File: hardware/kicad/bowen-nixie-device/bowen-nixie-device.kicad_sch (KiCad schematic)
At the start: 122 parts, among them J1 Conn_01x02_Pin, J2 Conn_01x02_Pin, J3 Conn_01x04_Pin, J4 Qwiic/Stemma QT, J5 Conn_01x03_Pin, Q1 MMBTA42, Q10 MMBTA42, Q11 MMBTA42, Q12 MMBTA42, Q13 MMBTA42, Q14 MMBTA42, Q15 MMBTA42, Q16 MMBTA42, Q17 MMBTA42, Q18 MMBTA42, Q19 MMBTA42, Q2 MMBTA92, Q20 MMBTA42, Q21 MMBTA42, Q22 MMBTA42, Q23 MMBTA42, Q24 MMBTA42, Q25 MMBTA42, Q26 MMBTA42, Q27 MMBTA42, Q28 MMBTA42, Q29 MMBTA42, Q3 MMBTA42, Q30 MMBTA42, Q31 MMBTA42, Q32 MMBTA42, Q33 MMBTA42, Q34 MMBTA42, Q35 MMBTA42, Q36 MMBTA42, Q37 MMBTA42, Q38 MMBTA42, Q39 MMBTA42, Q4 MMBTA92, Q40 MMBTA42, Q41 MMBTA42, Q42 MMBTA42, Q43 MMBTA42, Q44 MMBTA42, Q45 MMBTA42, Q46 MMBTA42, Q47 MMBTA42, Q48 MMBTA42, Q5 MMBTA42, Q6 MMBTA92, Q7 MMBTA42, Q8 MMBTA92, Q9 MMBTA42, U1 MOUDLE-SEEEDUINO-XIAO-ESP32C3, U11 NCH8200HV, U12 DS3231, U2 74HC595, U3 74HC595, U4 74HC595, U5 74HC595, U6 74HC595

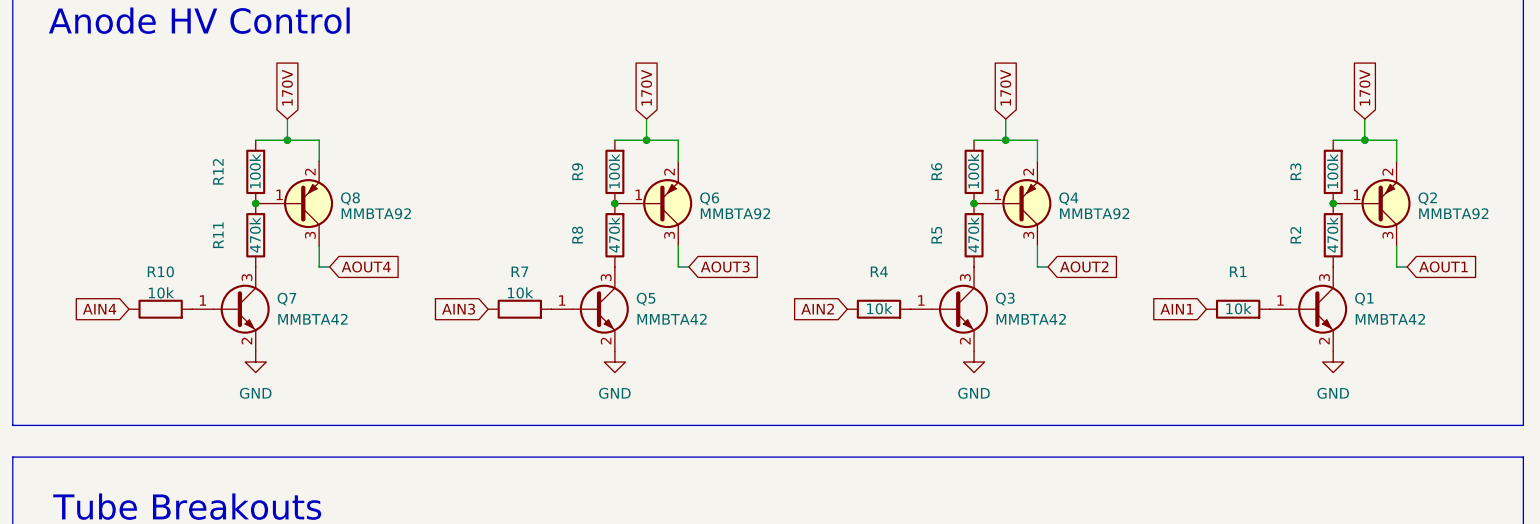
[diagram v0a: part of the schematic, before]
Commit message: bowen fixes, final v1
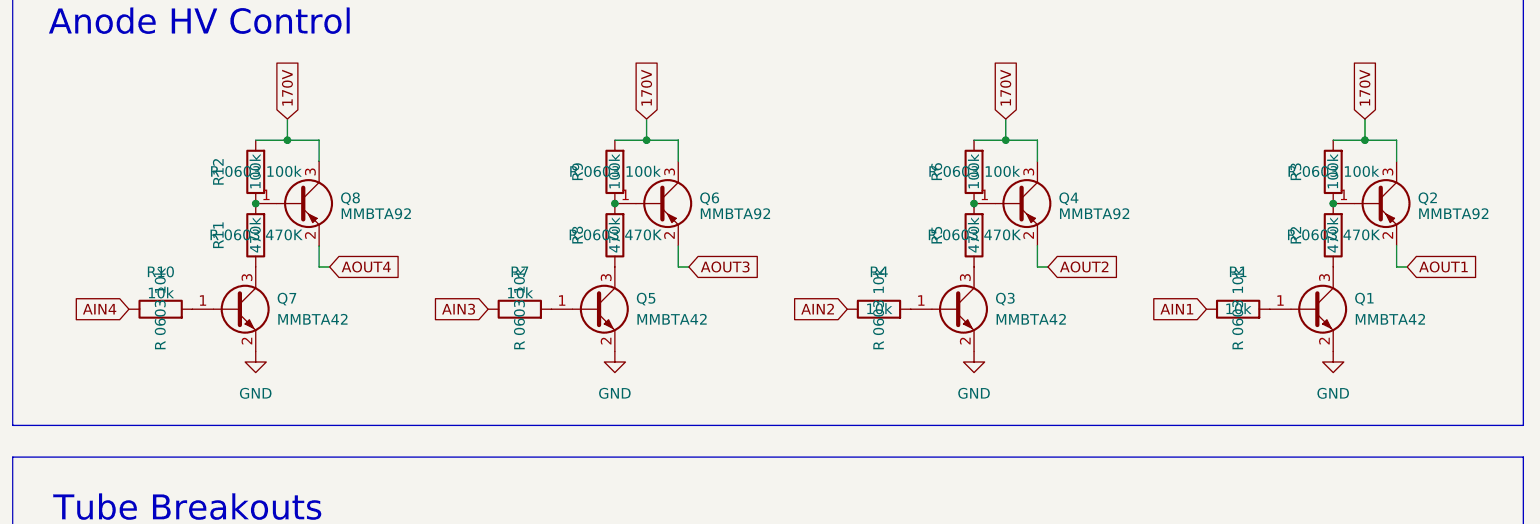
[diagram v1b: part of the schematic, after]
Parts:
- J4: MPN (none) -> BM04B-SRSS-TB
- Q1, Q10, Q11, Q12, Q13, Q14, Q15, Q16, Q17, Q18, Q19, Q20, Q21, Q22, Q23, Q24, Q25, Q26, Q27, Q28, Q29, Q3, Q30, Q31, Q32, Q33, Q34, Q35, Q36, Q37, Q38, Q39, Q40, Q41, Q42, Q43, Q44, Q45, Q46, Q47, Q48, Q5, Q7, Q9: MPN (none) -> MMBTA42LT1G; Package (none) -> SOT-23
- Q2, Q4, Q6, Q8: footprint PCM_Package_TO_SOT_SMD_AKL:SOT-23 -> Package_TO_SOT_SMD:SOT-23; symbol PCM_Transistor_BJT_AKL:MMBTA92 -> Transistor_BJT:MMBTA92; MPN (none) -> MMBTA92LT1G; Package (none) -> SOT-23
- R1, R10, R13, R14, R15, R16, R17, R18, R19, R20, R21, R22, R23, R24, R25, R26, R27, R28, R29, R30, R31, R32, R33, R34, R35, R36, R37, R38, R39, R4, R40, R41, R42, R43, R44, R45, R46, R47, R48, R49, R50, R51, R52, R7: MPN (none) -> RC0603JR-0710KL; Package (none) -> 0603
- R11, R2, R5, R8: MPN (none) -> RC1206FR-07470KL; Package (none) -> 1206
- R12, R3, R6, R9: MPN (none) -> RC0402FR-07100KL; Package (none) -> 0603
- U11: now in the parts list
- U2, U3, U4, U5, U6: MPN (none) -> 74HC595D; Package (none) -> SOIC-16
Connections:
- net 170V: now also Q2.3 (C), Q4.3 (C), Q6.3 (C), Q8.3 (C); no longer Q2.2 (E), Q4.2 (E), Q6.2 (E), Q8.2 (E)
- net AOUT1: now also Q2.2 (E); no longer Q2.3 (C)
- net AOUT2: now also Q4.2 (E); no longer Q4.3 (C)
- net AOUT3: now also Q6.2 (E); no longer Q6.3 (C)
- net AOUT4: now also Q8.2 (E); no longer Q8.3 (C)
